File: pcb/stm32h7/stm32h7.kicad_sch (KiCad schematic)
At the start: 39 parts, among them J6 Test Pads, SW1 SW_Push, SW2 SW_Push, SW3 SW_Push, U1 STM32H743VGTx, U11 TPS61169DCKR, U9 MT25QUxxxxxx1xW7, Y1 25MHz

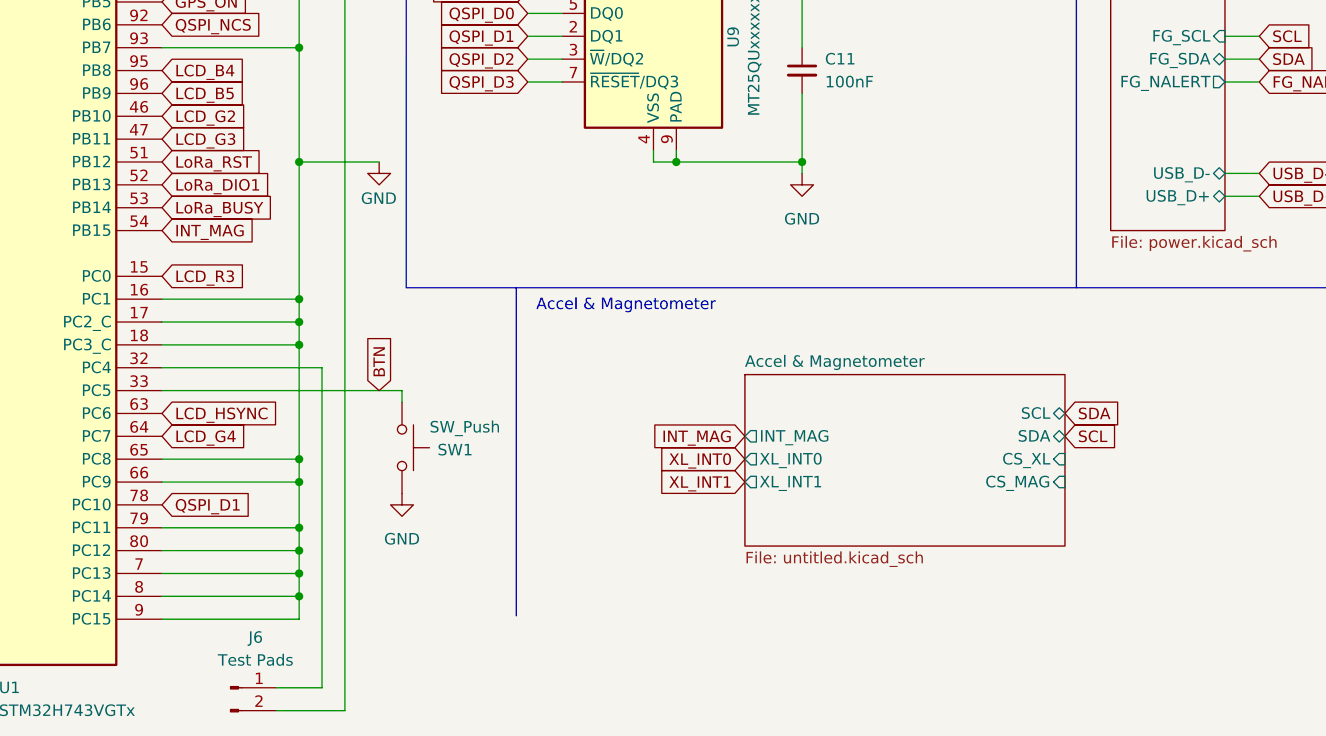
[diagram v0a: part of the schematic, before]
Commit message: is it finally done or am i going insane
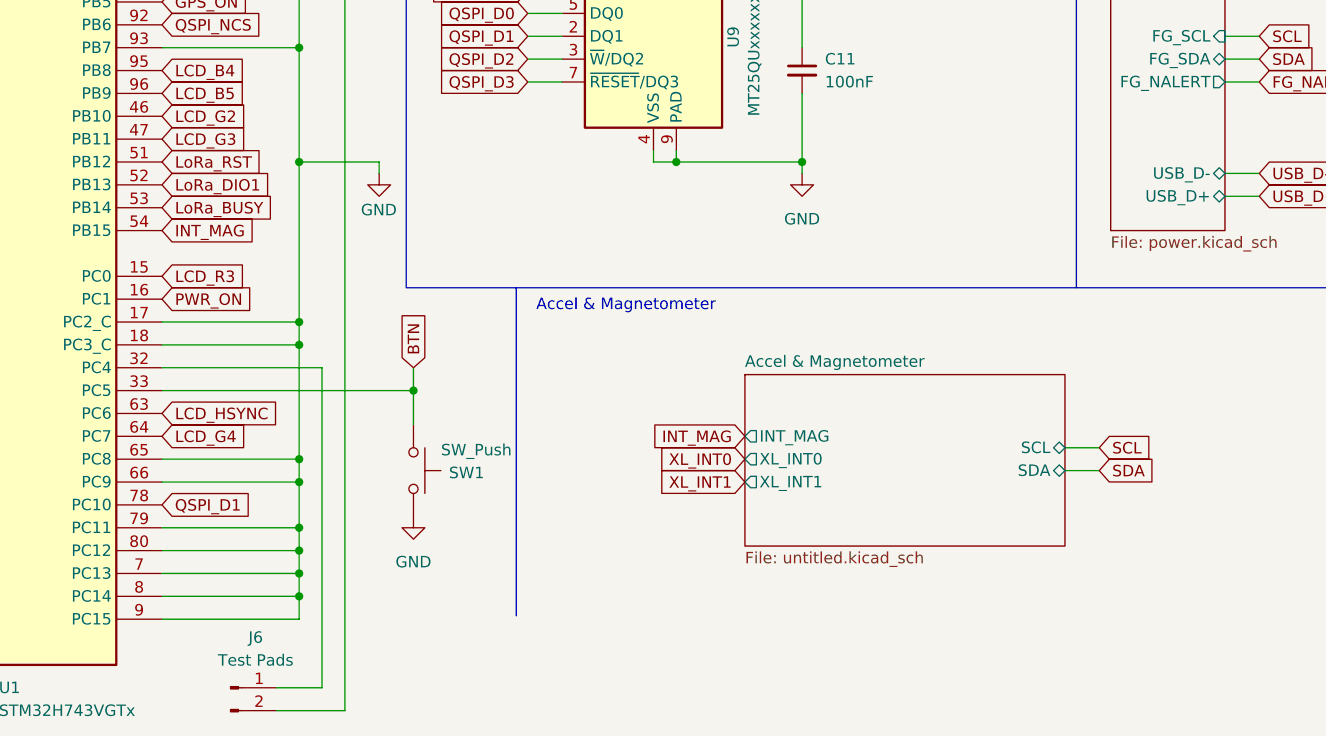
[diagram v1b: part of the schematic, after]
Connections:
- net GND: no longer U1.16 (PC1)
- new net PWR_ON: U1.16 (PC1)
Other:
- sheet Accel & Magnetometer ports: added none; removed CS_MAG, CS_XL
- moved on the sheet: SW1
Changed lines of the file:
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@@
 	)
 	(junction
-		(at 165.1 130.81)
-		(diameter 0)
-		(color 0 0 0 0)
-	)
-	(junction
 		(at 110.49 190.5)
 		(diameter 0)
@@
 	)
 	(junction
-		(at 165.1 163.83)
+		(at 177.8 140.97)
 		(diameter 0)
 		(color 0 0 0 0)
 	)
 	(junction
-		(at 228.6 31.75)
+		(at 165.1 163.83)
 		(diameter 0)
 		(color 0 0 0 0)
 	)
 	(junction
-		(at 87.63 185.42)
+		(at 228.6 31.75)
 		(diameter 0)
 		(color 0 0 0 0)
 	)
 	(junction
-		(at 165.1 115.57)
+		(at 87.63 185.42)
 		(diameter 0)
 		(color 0 0 0 0)
@@
 		(color 0 0 0 0)
 	)
+	(junction
+		(at 165.1 115.57)
+		(diameter 0)
+		(color 0 0 0 0)
+	)
 	(no_connect
 		(at 29.21 38.1)
@@
 	(wire
 		(pts
-			(xy 149.86 130.81) (xy 165.1 130.81)
-		)
-		(stroke
-			(width 0)
-			(type default)
-		)
-	)
-	(wire
-		(pts
 			(xy 104.14 34.29) (xy 104.14 38.1)
 		)
@@
 	(wire
 		(pts
-			(xy 165.1 130.81) (xy 165.1 133.35)
+			(xy 173.99 115.57) (xy 173.99 116.84)
 		)
 		(stroke
@@
 	(wire
 		(pts
+			(xy 165.1 115.57) (xy 165.1 133.35)
+		)
+		(stroke
+			(width 0)
+			(type default)
+		)
+	)
+	(wire
+		(pts
 			(xy 22.86 193.04) (xy 31.75 193.04)
 		)
@@
 	(wire
 		(pts
-			(xy 165.1 115.57) (xy 165.1 130.81)
-		)
-		(stroke
-			(width 0)
-			(type default)
-		)
-	)
-	(wire
-		(pts
 			(xy 144.78 190.5) (xy 156.21 190.5)
 		)
@@
 	(wire
 		(pts
+			(xy 177.8 140.97) (xy 177.8 138.43)
+		)
+		(stroke
+			(width 0)
+			(type default)
+		)
+	)
+	(wire
+		(pts
 			(xy 149.86 163.83) (xy 165.1 163.83)
 		)
@@
 	(wire
 		(pts
+			(xy 250.19 147.32) (xy 254 147.32)
+		)
+		(stroke
+			(width 0)
+			(type default)
+		)
+	)
+	(wire
+		(pts
 			(xy 95.25 163.83) (xy 95.25 165.1)
 		)
@@
 	(wire
 		(pts
+			(xy 149.86 140.97) (xy 177.8 140.97)
+		)
+		(stroke
+			(width 0)
+			(type default)
+		)
+	)
+	(wire
+		(pts
 			(xy 100.33 163.83) (xy 100.33 160.02)
 		)
@@
 	(wire
 		(pts
-			(xy 176.53 142.24) (xy 176.53 140.97)
+			(xy 177.8 144.78) (xy 177.8 140.97)
+		)
+		(stroke
+			(width 0)
+			(type default)
+		)
+	)
+	(wire
+		(pts
+			(xy 250.19 149.86) (xy 254 149.86)
 		)
 		(stroke
@@
 	(wire
 		(pts
-			(xy 149.86 140.97) (xy 176.53 140.97)
-		)
-		(stroke
-			(width 0)
-			(type default)
-		)
-	)
-	(wire
-		(pts
 			(xy 30.48 177.8) (xy 30.48 181.61)
 		)
@@
 	(global_label "SCL"
 		(shape input)
-		(at 250.19 146.05 0)
+		(at 254 147.32 0)
 		(fields_autoplaced yes)
 		(effects
@@
 		)
 		(property "Intersheetrefs" "${INTERSHEET_REFS}"
-			(at 256.6828 146.05 0)
+			(at 260.4928 147.32 0)
 			(effects
 				(font
@@
 		)
 	)
+	(global_label "PWR_ON"
+		(shape input)
+		(at 149.86 130.81 0)
+		(fields_autoplaced yes)
+		(effects
+			(font
+				(size 1.27 1.27)
+			)
+			(justify left)
+		)
+		(property "Intersheetrefs" "${INTERSHEET_REFS}"
+			(at 160.4652 130.81 0)
+			(effects
+				(font
+					(size 1.27 1.27)
+				)
+				(justify left)
+				(hide yes)
+			)
+		)
+	)
 	(global_label "LCD_CS"
 		(shape input)
@@
 	(global_label "SDA"
 		(shape input)
-		(at 250.19 143.51 0)
+		(at 254 149.86 0)
 		(fields_autoplaced yes)
 		(effects
@@
 		)
 		(property "Intersheetrefs" "${INTERSHEET_REFS}"
-			(at 256.7433 143.51 0)
+			(at 260.5533 149.86 0)
 			(effects
 				(font
@@
 	(global_label "BTN"
 		(shape input)
-		(at 173.99 140.97 90)
+		(at 177.8 138.43 90)
 		(fields_autoplaced yes)
 		(effects
@@
 		)
 		(property "Intersheetrefs" "${INTERSHEET_REFS}"
-			(at 173.99 134.4167 90)
+			(at 177.8 131.8767 90)
 			(effects
 				(font
@@
 	(symbol
 		(lib_id "Switch:SW_Push")
-		(at 176.53 147.32 270)
+		(at 177.8 149.86 270)
 		(unit 1)
 		(exclude_from_sim no)
@@
 		(dnp no)
 		(property "Reference" "SW1"
-			(at 184.404 147.574 90)
+			(at 185.674 150.114 90)
 			(effects
 				(font
@@
 		)
 		(property "Value" "SW_Push"
-			(at 187.452 145.034 90)
+			(at 188.722 147.574 90)
 			(effects
 				(font
@@
 		)
 		(property "Footprint" "custom_comps:vert_button_6mm"
-			(at 181.61 147.32 0)
+			(at 182.88 149.86 0)
 			(effects
 				(font
@@
 		)
 		(property "Datasheet" "~"
-			(at 181.61 147.32 0)
+			(at 182.88 149.86 0)
 			(effects
 				(font
@@
 		)
 		(property "Description" "Push button switch, generic, two pins"
-			(at 176.53 147.32 0)
+			(at 177.8 149.86 0)
 			(effects
 				(font
@@
 	(symbol
 		(lib_id "power:GND")
-		(at 176.53 152.4 0)
+		(at 177.8 154.94 0)
 		(unit 1)
 		(exclude_from_sim no)
@@
 		(fields_autoplaced yes)
 		(property "Reference" "#PWR082"
-			(at 176.53 158.75 0)
+			(at 177.8 161.29 0)
 			(effects
 				(font
@@
 		)
 		(property "Value" "GND"
-			(at 176.53 157.48 0)
+			(at 177.8 160.02 0)
 			(effects
 				(font
@@
 		)
 		(property "Footprint" ""
-			(at 176.53 152.4 0)
+			(at 177.8 154.94 0)
 			(effects
 				(font
@@
 		)
 		(property "Datasheet" ""
-			(at 176.53 152.4 0)
+			(at 177.8 154.94 0)
 			(effects
 				(font
@@
 		)
 		(property "Description" "Power symbol creates a global label with name \"GND\" , ground"
-			(at 176.53 152.4 0)
+			(at 177.8 154.94 0)
 			(effects
 				(font
@@
 	(symbol
 		(lib_id "power:GND")
-		(at 173.99 115.57 0)
+		(at 173.99 116.84 0)
 		(unit 1)
 		(exclude_from_sim no)
@@
 		(dnp no)
 		(property "Reference" "#PWR077"
-			(at 173.99 121.92 0)
+			(at 173.99 123.19 0)
 			(effects
 				(font
@@
 		)
 		(property "Value" "GND"
-			(at 171.958 119.634 0)
+			(at 171.958 120.904 0)
 			(effects
 				(font
@@
 		)
 		(property "Footprint" ""
-			(at 173.99 115.57 0)
+			(at 173.99 116.84 0)
 			(effects
 				(font
@@
 		)
 		(property "Datasheet" ""
-			(at 173.99 115.57 0)
+			(at 173.99 116.84 0)
 			(effects
 				(font
@@
 		)
 		(property "Description" "Power symbol creates a global label with name \"GND\" , ground"
-			(at 173.99 115.57 0)
+			(at 173.99 116.84 0)
 			(effects
 				(font
@@
 		)
 		(pin "SDA" bidirectional
-			(at 250.19 146.05 0)
+			(at 250.19 149.86 0)
 			(effects
 				(font
@@
 		)
 		(pin "SCL" bidirectional
-			(at 250.19 143.51 0)
+			(at 250.19 147.32 0)
 			(effects
 				(font
@@
 			)
 		)
-		(pin "CS_XL" input
-			(at 250.19 148.59 0)
-			(effects
-				(font
-					(size 1.27 1.27)
-				)
-				(justify right)
-			)
-		)
-		(pin "CS_MAG" input
-			(at 250.19 151.13 0)
-			(effects
-				(font
-					(size 1.27 1.27)
-				)
-				(justify right)
-			)
-		)
